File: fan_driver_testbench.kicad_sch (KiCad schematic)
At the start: 6 parts, among them Q5 BTS141

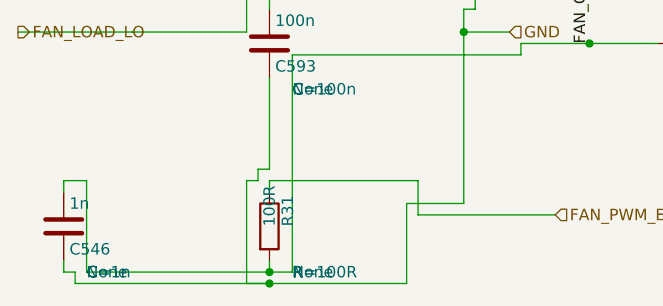
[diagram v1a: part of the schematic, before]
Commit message: fix
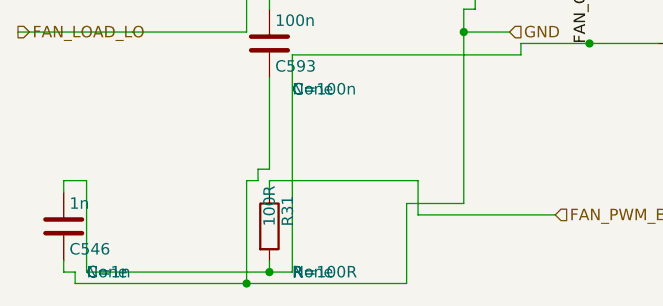
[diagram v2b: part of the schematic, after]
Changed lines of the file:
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@@
 				(instances
 			(project "climate_control_niva_travel"
-				(path "/9d65f2b6-eafc-4877-87dc-8b71e3390a39"(reference "R31") (unit 1) )
+				(path "/3bdb15f9-9517-4ddf-9f93-5c92d7358861"(reference "R31") (unit 1) )
 			)
 		)
@@
 				(instances
 			(project "climate_control_niva_travel"
-				(path "/9d65f2b6-eafc-4877-87dc-8b71e3390a39"(reference "C546") (unit 1) )
+				(path "/3bdb15f9-9517-4ddf-9f93-5c92d7358861"(reference "C546") (unit 1) )
 			)
 		)
@@
 				(instances
 			(project "climate_control_niva_travel"
-				(path "/9d65f2b6-eafc-4877-87dc-8b71e3390a39"(reference "Q5") (unit 1) )
+				(path "/3bdb15f9-9517-4ddf-9f93-5c92d7358861"(reference "Q5") (unit 1) )
 			)
 		)
@@
 				(instances
 			(project "climate_control_niva_travel"
-				(path "/9d65f2b6-eafc-4877-87dc-8b71e3390a39"(reference "D6") (unit 1) )
+				(path "/3bdb15f9-9517-4ddf-9f93-5c92d7358861"(reference "D6") (unit 1) )
 			)
 		)
@@
 				(instances
 			(project "climate_control_niva_travel"
-				(path "/9d65f2b6-eafc-4877-87dc-8b71e3390a39"(reference "L637") (unit 1) )
+				(path "/3bdb15f9-9517-4ddf-9f93-5c92d7358861"(reference "L637") (unit 1) )
 			)
 		)
@@
 				(instances
 			(project "climate_control_niva_travel"
-				(path "/9d65f2b6-eafc-4877-87dc-8b71e3390a39"(reference "C593") (unit 1) )
+				(path "/3bdb15f9-9517-4ddf-9f93-5c92d7358861"(reference "C593") (unit 1) )
 			)
 		)
@@
 		(pts
 			(xy 29.21 43.18) (xy 29.21 54.61)
-		)
-		(stroke
-			(width 0)
-			(type default)
-		)
-	)
-	(wire
-		(pts
-			(xy 29.21 54.61) (xy 31.75 54.61)
 		)
 		(stroke
@@
 	)
 	(junction
-		(at 31.75 54.61)
+		(at 29.21 54.61)
 		(diameter 0.0000)
 		(color 0 0 0 0)
